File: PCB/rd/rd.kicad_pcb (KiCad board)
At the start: 2 copper layers, 15 x 29.5 mm, 14 parts, among them U1 GL823K-HCY04

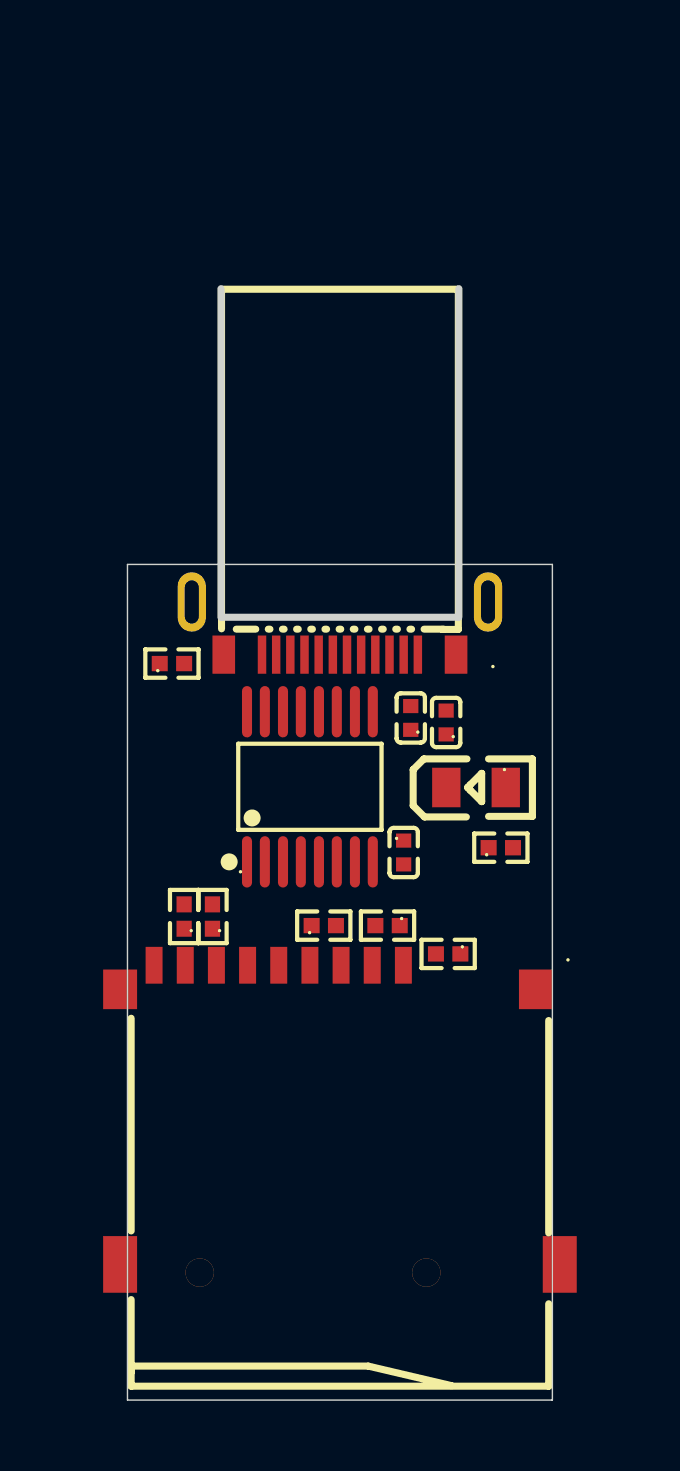
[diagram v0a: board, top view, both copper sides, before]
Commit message: routing
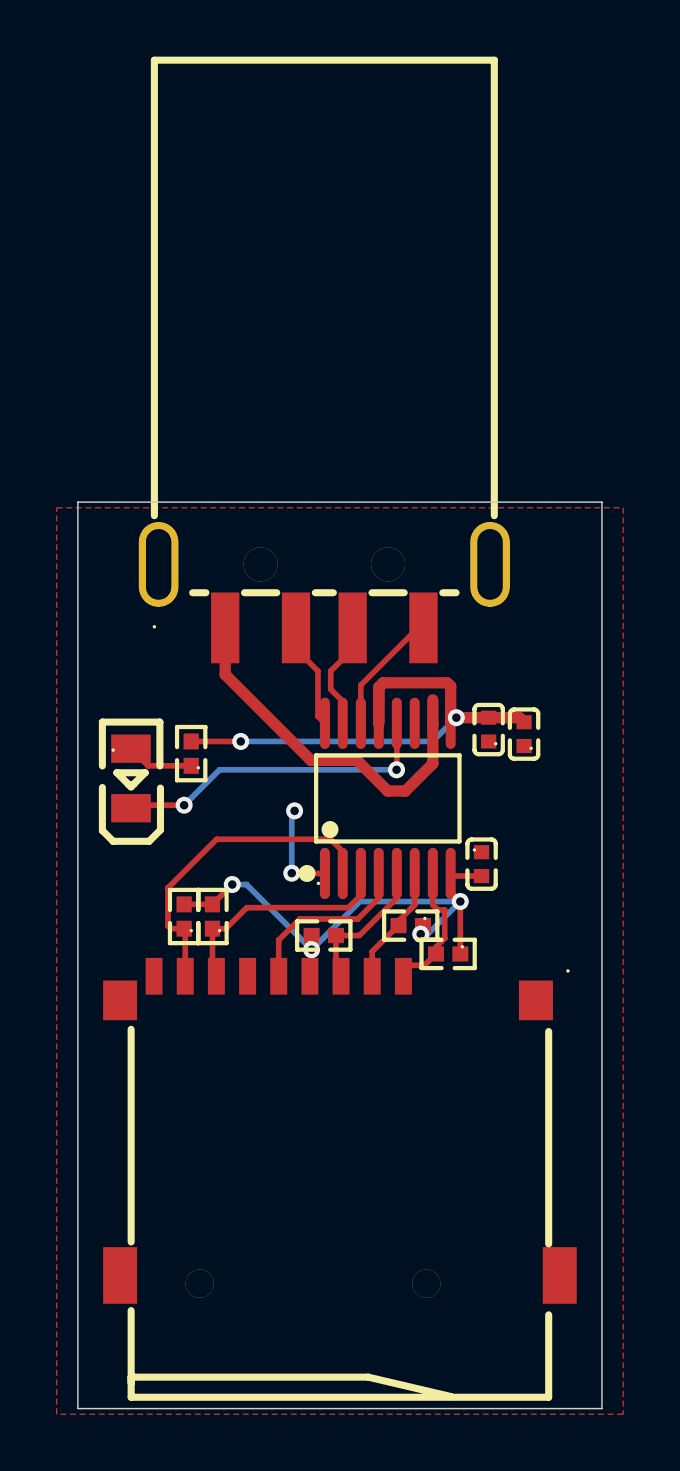
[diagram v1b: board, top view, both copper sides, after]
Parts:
- removed R2: 5.1k, easyeda2kicad:R0402
- USB1: value GT-USB-8016B -> U-USBAR04P-M001; footprint easyeda2kicad:USB-SMD_GT-USB-8016B -> easyeda2kicad:USB-SMD_KH-USB-AM-4P-CB
- moved LED1 12.2 mm to (72.6, 84.6), turned to 90 degrees
- moved R1 11.4 mm to (74.8, 83.7), turned to 90 degrees
- moved U1 2.78 mm to (81.7, 85.3)
- moved C1 2.78 mm to (85.2, 82.8)
- moved C2 2.78 mm to (85.0, 87.6)
- moved C3 2.78 mm to (86.5, 83.0)
- moved USB1 1.26 mm to (79.5, 78.1)
- moved R11 0.82 mm to (82.5, 89.8)
- moved Card1 0.39 mm to (80.0, 96.8)
- moved R9 0.35 mm to (79.4, 90.1)
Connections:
- USB1 pad 1: GND -> /VBUS
- USB1 pad 2: GND -> /D-
- USB1 pad 3: GND -> /D+
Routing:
- net /PMOS: track 0.00 -> 19.0 mm, vias 0 -> 4
- net /VDD: track 0.00 -> 18.8 mm, vias 0 -> 2
- net /VBUS: track 0.00 -> 13.3 mm
- net /LED: track 0.00 -> 11.6 mm, vias 0 -> 2
- net /D1: track 0.00 -> 11.1 mm
- net /D0: track 0.00 -> 7.84 mm
- net GND: track 0.00 -> 7.81 mm, vias 0 -> 2
- net /CLK: track 0.00 -> 5.90 mm
- net /CMD: track 0.00 -> 4.69 mm
- net /D2: track 0.00 -> 4.60 mm
- net /D3: track 0.00 -> 4.10 mm
- net /D+: track 0.00 -> 3.87 mm
- net /D-: track 0.00 -> 3.79 mm
- net Net-(LED1-A): track 0.00 -> 2.38 mm
- added copper zone on F.Cu, net GND
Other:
- board size 15 x 29.5 mm -> 18.5 x 32 mm
